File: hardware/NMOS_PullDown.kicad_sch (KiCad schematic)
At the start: 3 parts, among them Q4 2N7002

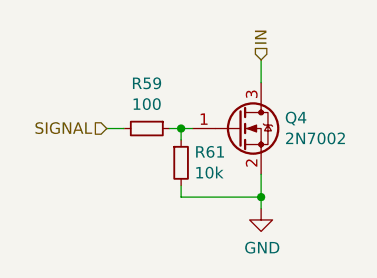
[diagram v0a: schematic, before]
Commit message: sync
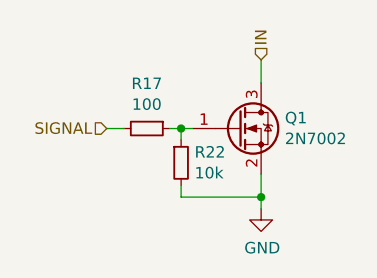
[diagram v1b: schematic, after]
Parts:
- renumbered Q4 to Q1, R59 to R17, R61 to R22
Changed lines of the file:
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@@
   (symbol (lib_id "Transistor_FET:2N7002") (at 145.415 94.615 0)
     (in_bom yes) (on_board yes)
-    (property "Reference" "Q4" (id 0) (at 150.5966 93.4466 0)
+    (property "Reference" "Q1" (id 0) (at 150.5966 93.4466 0)
       (effects (font (size 1.27 1.27)) (justify left))
     )
@@
   (symbol (lib_id "Device:R_Small") (at 139.065 98.425 0)
     (in_bom yes) (on_board yes)
-    (property "Reference" "R61" (id 0) (at 140.5636 97.2566 0)
+    (property "Reference" "R22" (id 0) (at 140.5636 97.2566 0)
       (effects (font (size 1.27 1.27)) (justify left))
     )
@@
   (symbol (lib_id "Device:R_Small") (at 135.255 94.615 270)
     (in_bom yes) (on_board yes)
-    (property "Reference" "R59" (id 0) (at 135.255 89.6366 90))
+    (property "Reference" "R17" (id 0) (at 135.255 89.6366 90))
     (property "Value" "100" (id 1) (at 135.255 91.948 90))
     (property "Footprint" "Resistor_SMD:R_0603_1608Metric" (id 2) (at 135.255 94.615 0)
